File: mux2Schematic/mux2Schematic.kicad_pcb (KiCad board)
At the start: 2 copper layers, 215 x 58 mm, 64 parts, among them J1 Conn_02x12_Odd_Even, J10 Conn_02x06_Top_Bottom, J11 Conn_02x06_Top_Bottom, J12 Conn_02x06_Top_Bottom, J13 Conn_02x06_Top_Bottom, J14 Conn_02x06_Top_Bottom, J15 Conn_01x02, J16 Conn_01x02, J17 Conn_01x02, J18 Conn_01x02, J19 Conn_01x02, J2 Conn_02x06_Top_Bottom, J20 Conn_01x02, J21 Conn_01x02, J3 Banana, J30 Conn_01x8, J31 Conn_01x8, J32 Conn_01x02, J33 Conn_01x02, J34 Conn_01x02, J35 Conn_01x02, J36 Conn_01x02, J37 Conn_01x02, J38 Conn_01x02, J39 Conn_01x02, J4 Banana, J5 Conn_01x8, J6 Conn_01x02, J7 Conn_02x06_Top_Bottom, J8 Conn_01x10, J9 Conn_02x06_Top_Bottom, U1 CD74HC4051E, U2 AMS1117-1.8, U3 AZ1084-3.3

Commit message: minor tweaks to PCB
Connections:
- J1 pad 10: unconnected-(J1-Pin_10-Pad10) -> /~{LDAC}
- J1 pad 12: unconnected-(J1-Pin_12-Pad12) -> /SCLK
- J1 pad 16: unconnected-(J1-Pin_16-Pad16) -> /CIPO
- J1 pad 18: unconnected-(J1-Pin_18-Pad18) -> /COPI
- J1 pad 19: unconnected-(J1-Pin_19-Pad19) -> /CS
- J1 pad 21: unconnected-(J1-Pin_21-Pad21) -> /S2
- J1 pad 22: unconnected-(J1-Pin_22-Pad22) -> /S0
- J1 pad 24: unconnected-(J1-Pin_24-Pad24) -> /S1
- J1 pad 4: unconnected-(J1-Pin_4-Pad4) -> /~{CLR}
- J1 pad 6: unconnected-(J1-Pin_6-Pad6) -> /~{RESET}

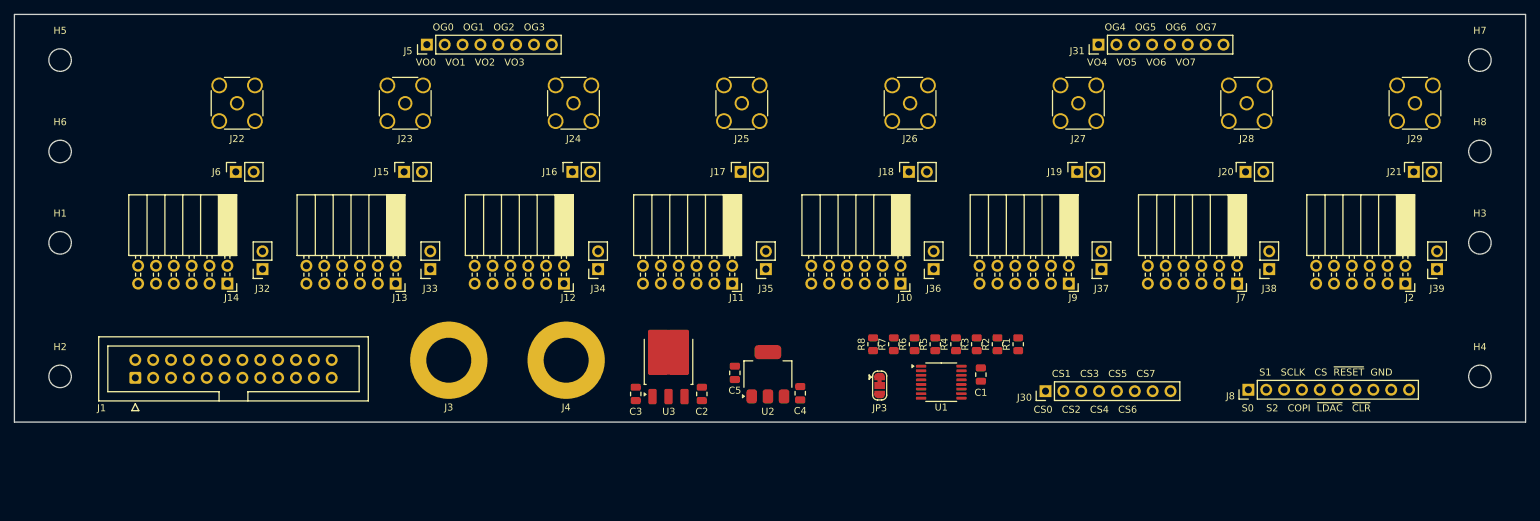
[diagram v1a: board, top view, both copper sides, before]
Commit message: PCB finished!
Haven't thoroughly looked it over yet
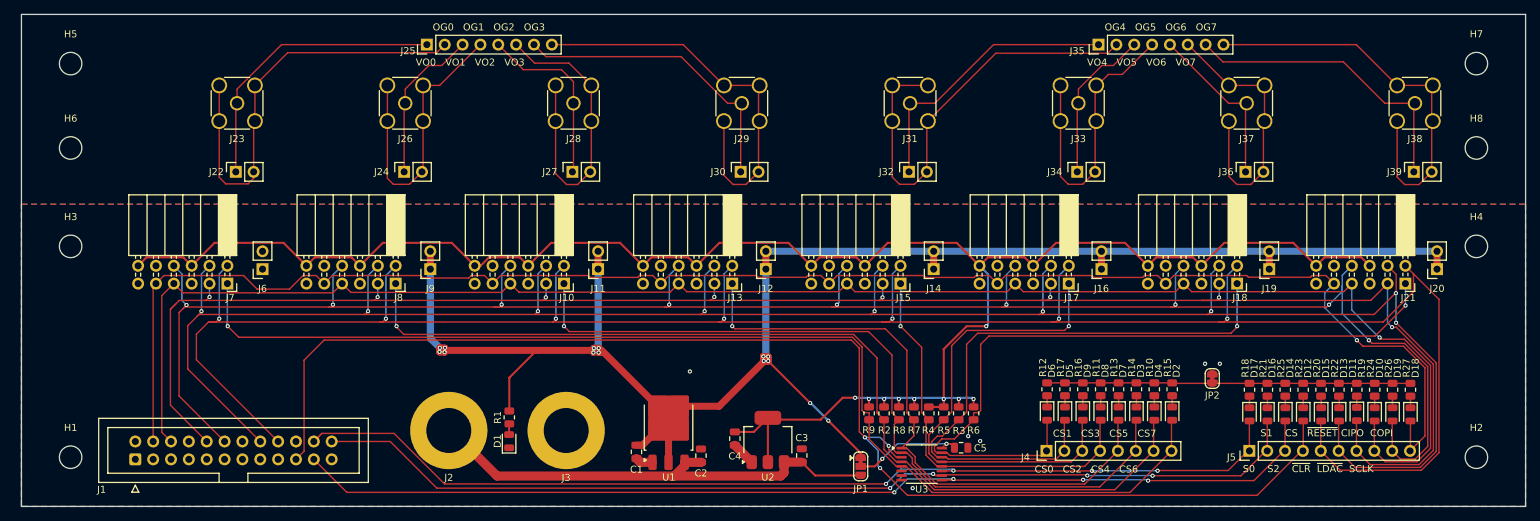
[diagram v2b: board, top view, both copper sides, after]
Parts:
- added D1: HSMA-C170, LED_SMD:LED_0805_2012Metric, F.Cu at (116.4, 146.7)
- added D10: HSMA-C170, LED_SMD:LED_0805_2012Metric, F.Cu at (239.5, 142.9)
- added D11: HSMA-C170, LED_SMD:LED_0805_2012Metric, F.Cu at (237.0, 142.9)
- added D12: HSMA-C170, LED_SMD:LED_0805_2012Metric, F.Cu at (229.4, 142.9)
- added D13: HSMA-C170, LED_SMD:LED_0805_2012Metric, F.Cu at (234.5, 142.9)
- added D14: HSMA-C170, LED_SMD:LED_0805_2012Metric, F.Cu at (226.8, 142.9)
- added D15: HSMA-C170, LED_SMD:LED_0805_2012Metric, F.Cu at (231.9, 142.9)
- added D16: HSMA-C170, LED_SMD:LED_0805_2012Metric, F.Cu at (224.3, 142.9)
- added D17: HSMA-C170, LED_SMD:LED_0805_2012Metric, F.Cu at (221.7, 142.9)
- added D18: HSMA-C170, LED_SMD:LED_0805_2012Metric, F.Cu at (244.6, 142.9)
- added D19: HSMA-C170, LED_SMD:LED_0805_2012Metric, F.Cu at (242.1, 142.9)
- added D2: HSMA-C170, LED_SMD:LED_0805_2012Metric, F.Cu at (210.7, 142.8)
- added D3: HSMA-C170, LED_SMD:LED_0805_2012Metric, F.Cu at (205.6, 142.8)
- added D4: HSMA-C170, LED_SMD:LED_0805_2012Metric, F.Cu at (208.2, 142.8)
- added D5: HSMA-C170, LED_SMD:LED_0805_2012Metric, F.Cu at (195.5, 142.8)
- added D6: HSMA-C170, LED_SMD:LED_0805_2012Metric, F.Cu at (192.9, 142.8)
- added D7: HSMA-C170, LED_SMD:LED_0805_2012Metric, F.Cu at (203.1, 142.8)
- added D8: HSMA-C170, LED_SMD:LED_0805_2012Metric, F.Cu at (200.5, 142.8)
- added D9: HSMA-C170, LED_SMD:LED_0805_2012Metric, F.Cu at (198.0, 142.8)
- added JP2: SolderJumper_2_Bridged, Jumper:SolderJumper-2_P1.3mm_Bridged_RoundedPad1.0x1.5mm, F.Cu at (216.4, 137.8)
- added R1: 5.1k, Resistor_SMD:R_0805_2012Metric, F.Cu at (116.4, 143.3)
- added R10: 2.2k, Resistor_SMD:R_0805_2012Metric, F.Cu at (208.2, 139.3)
- added R11: 2.2k, Resistor_SMD:R_0805_2012Metric, F.Cu at (200.5, 139.3)
- added R12: 2.2k, Resistor_SMD:R_0805_2012Metric, F.Cu at (192.9, 139.3)
- added R13: 2.2k, Resistor_SMD:R_0805_2012Metric, F.Cu at (203.1, 139.3)
- added R14: 2.2k, Resistor_SMD:R_0805_2012Metric, F.Cu at (205.6, 139.3)
- added R15: 2.2k, Resistor_SMD:R_0805_2012Metric, F.Cu at (210.7, 139.3)
- added R16: 2.2k, Resistor_SMD:R_0805_2012Metric, F.Cu at (198.0, 139.3)
- added R17: 2.2k, Resistor_SMD:R_0805_2012Metric, F.Cu at (195.5, 139.3)
- added R18: 2.2k, Resistor_SMD:R_0805_2012Metric, F.Cu at (221.7, 139.4)
- added R19: 2.2k, Resistor_SMD:R_0805_2012Metric, F.Cu at (237.0, 139.4)
- added R20: 2.2k, Resistor_SMD:R_0805_2012Metric, F.Cu at (231.9, 139.4)
- added R21: 2.2k, Resistor_SMD:R_0805_2012Metric, F.Cu at (224.3, 139.4)
- added R22: 2.2k, Resistor_SMD:R_0805_2012Metric, F.Cu at (234.4, 139.4)
- added R23: 2.2k, Resistor_SMD:R_0805_2012Metric, F.Cu at (229.4, 139.4)
- added R24: 2.2k, Resistor_SMD:R_0805_2012Metric, F.Cu at (239.5, 139.4)
- added R25: 2.2k, Resistor_SMD:R_0805_2012Metric, F.Cu at (226.8, 139.4)
- added R26: 2.2k, Resistor_SMD:R_0805_2012Metric, F.Cu at (242.1, 139.4)
- added R27: 2.2k, Resistor_SMD:R_0805_2012Metric, F.Cu at (244.6, 139.4)
- R2: renamed from R7; value 10k -> 5.1k
- R3: renamed from R2; value 10k -> 5.1k
- R4: value 10k -> 5.1k
- R5: renamed from R3; value 10k -> 5.1k
- R6: renamed from R1; value 10k -> 5.1k
- R7: renamed from R5; value 10k -> 5.1k
- R8: renamed from R6; value 10k -> 5.1k
- R9: renamed from R8; value 10k -> 5.1k
- moved J10 23.9 mm to (124.2, 124.3)
- moved J8 23.9 mm to (100.2, 124.3)
- moved U3 12.0 mm to (175.1, 150.0)
- moved JP1 11.8 mm to (166.4, 150.3)
- moved R6 11.7 mm to (182.5, 142.8)
- moved J1 11.6 mm to (63.2, 149.3)
- moved H1 11.6 mm to (54.0, 149.0)
- moved H2 11.5 mm to (254.0, 149.0)
- moved R3 11.3 mm to (180.3, 142.8)
- moved R5 10.9 mm to (178.2, 142.8)
- moved C5 10.8 mm to (180.7, 147.7), turned to 0 degrees
- moved R4 10.6 mm to (176.1, 142.8)
- moved R7 10.3 mm to (174.0, 142.8)
- moved R8 10.1 mm to (171.8, 142.8)
- moved J2 10.0 mm to (107.8, 145.2)
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- renumbered C3 to C1, C4 to C3, C5 to C4, C1 to C5, H2 to H1, H4 to H2, H1 to H3, H3 to H4, J13 to J10, J34 to J11, J35 to J12, J11 to J13, J36 to J14, J10 to J15, J37 to J16, J9 to J17, J7 to J18, J38 to J19, J3 to J2, J39 to J20, J2 to J21, J6 to J22, J22 to J23, J15 to J24, J5 to J25, J23 to J26, J16 to J27, J24 to J28, J25 to J29, J4 to J3, J17 to J30, J26 to J31, J18 to J32, J27 to J33, J19 to J34, J31 to J35, J20 to J36, J28 to J37, J29 to J38, J21 to J39, J30 to J4, J8 to J5, J32 to J6, J14 to J7, J12 to J8, J33 to J9, JP3 to JP1, U3 to U1, U1 to U3
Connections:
- J1 pad 10: /~{LDAC} -> /CIPO
- J1 pad 12: /SCLK -> /~{RESET}
- J1 pad 16: /CIPO -> /SCLK
- J1 pad 6: /~{RESET} -> /~{LDAC}
- J5 pad 10: GND -> /~{CLR}
- J5 pad 4: /SCLK -> /CS
- J5 pad 6: /CS -> /SCLK
- J5 pad 7: /~{LDAC} -> /CIPO
- J5 pad 8: /~{RESET} -> /~{LDAC}
- J5 pad 9: /~{CLR} -> /~{RESET}
- U3 pad 13: /CS_0 -> /CS_2
- U3 pad 15: /CS_2 -> /CS_0
- U3 pad 2: /CS_6 -> /CS_5
- U3 pad 4: /CS_7 -> /CS_6
- U3 pad 5: /CS_5 -> /CS_7
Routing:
- net /COPI: track 0.00 -> 315.2 mm, vias 0 -> 7
- net /SCLK: track 0.00 -> 298.4 mm, vias 0 -> 9
- net /~{RESET}: track 0.00 -> 281.7 mm, vias 0 -> 9
- net /IOVcc: track 0.00 -> 279.4 mm, vias 0 -> 9
- net /CIPO: track 0.00 -> 263.0 mm, vias 0 -> 8
- net /VCC: track 0.00 -> 247.3 mm, vias 0 -> 14
- net /~{LDAC}: track 0.00 -> 242.0 mm, vias 0 -> 1
- net /~{CLR}: track 0.00 -> 239.0 mm, vias 0 -> 1
- net /CS: track 0.00 -> 189.3 mm, vias 0 -> 3
- net /CS_7: track 0.00 -> 165.1 mm, vias 0 -> 1
- net /S2: track 0.00 -> 149.1 mm, vias 0 -> 4
- net /S0: track 0.00 -> 146.4 mm, vias 0 -> 4
- net /S1: track 0.00 -> 142.9 mm, vias 0 -> 4
- net /CS_6: track 0.00 -> 137.4 mm, vias 0 -> 1
- net /CS_5: track 0.00 -> 112.2 mm, vias 0 -> 1
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- added copper zone on B.Cu, net GND
- added copper zone on F.Cu, net GND
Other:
- board size 215 x 58 mm -> 214 x 70 mm
- board text added: "S0 S2 ~{CLR} ~{LDAC} SCLK"
- board text added: "S1 CS ~{RESET} CIPO COPI"
- board text added: "add an IDC for DAC out for Prototype 2"
- board text removed: "Are there any signals sensitive to parasitic inductance from vias?"
- board text removed: "S0 S2 COPI ~{LDAC} ~{CLR}"
- board text removed: "S1 SCLK CS ~{RESET} GND"
- board text removed: "add another IDC on DAC out for P2"
- board text removed: "add silkscree"
- board text removed: "add silkscreen"
- board text removed: "and LEDs"
- board text removed: "is this plated hole footprint for the bananas good?"
- board text removed: "split into two PCBs"
